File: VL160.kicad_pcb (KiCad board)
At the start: 4 copper layers, 24 x 14 mm, 12 parts, among them J1 USB_C_Receptacle, J2 USB3_A, U1 VL160, U2 LM3480-5.0

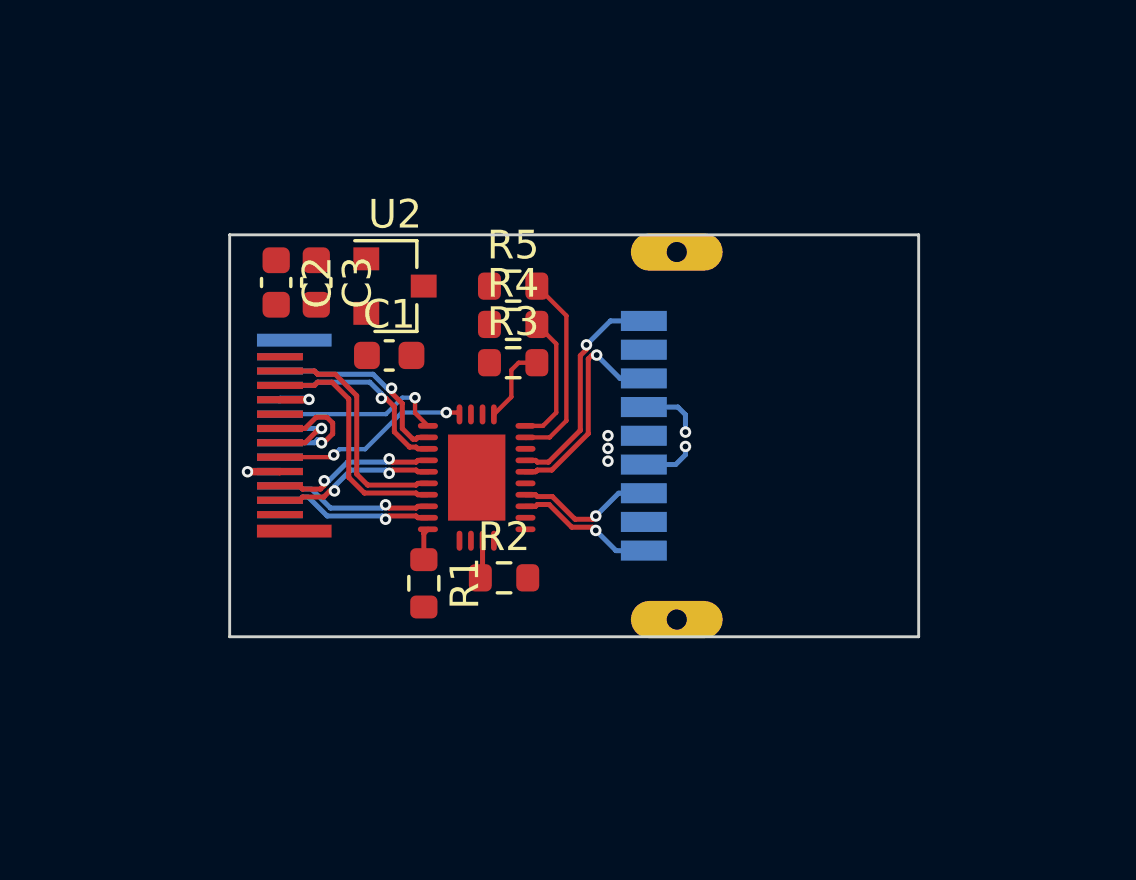
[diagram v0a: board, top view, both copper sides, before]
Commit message: Sync 2022/01/11 周二 21:14:02.89
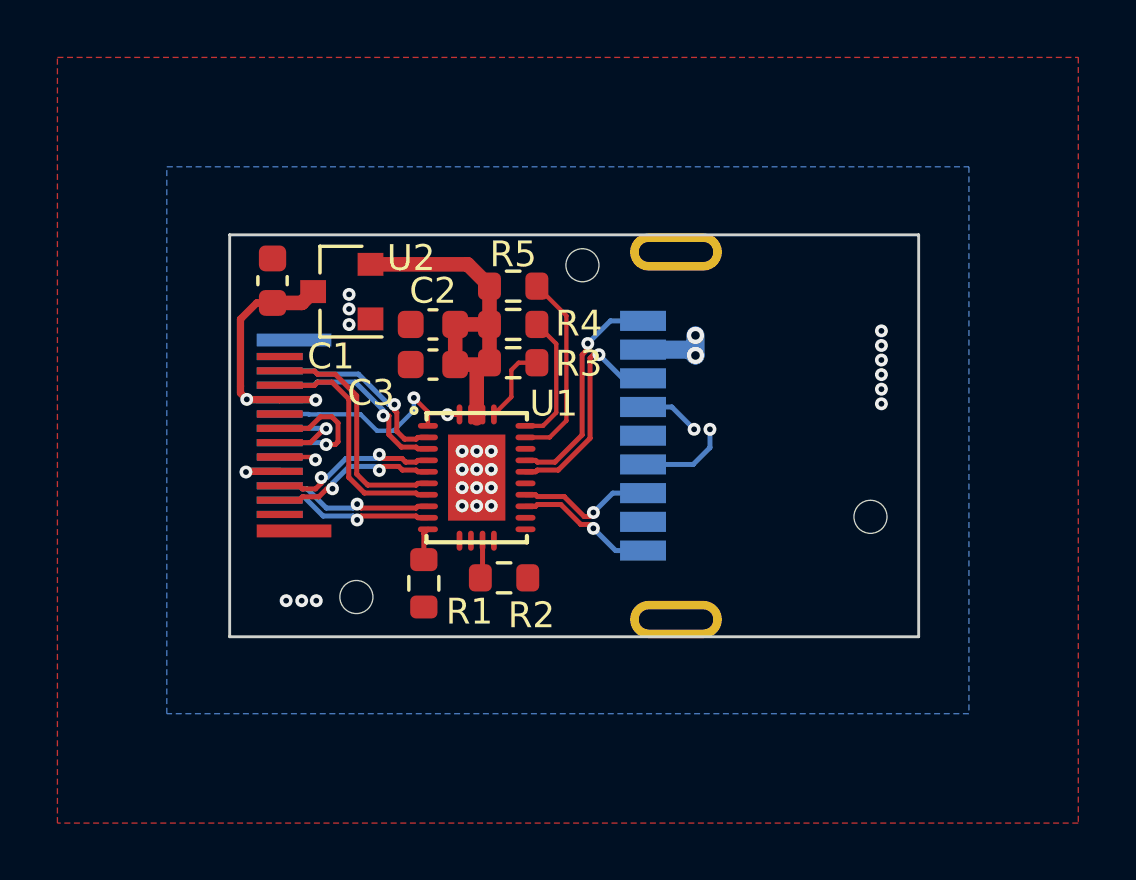
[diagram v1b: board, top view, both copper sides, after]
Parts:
- added H1: MountingHole, VL160:Hole_1.152mm_JLCSMT, F.Cu at (137.4, 102.6)
- added H2: MountingHole, VL160:Hole_1.152mm_JLCSMT, F.Cu at (155.3, 99.8)
- added H3: MountingHole, VL160:Hole_1.152mm_JLCSMT, F.Cu at (145.3, 91.1)
- J1, J2: moved to B.Cu
- U2: value LM3480-5.0 -> SE8550
- moved C2 5.65 mm to (140.1, 93.1), turned to 180 degrees
- moved C3 4.97 mm to (140.1, 94.5), turned to 180 degrees
- moved C1 4.83 mm to (134.5, 91.6), turned to 90 degrees
- moved J1 3.39 mm to (135.2, 93.6)
- moved U2 1.86 mm to (136.9, 92.0), turned to 180 degrees
- moved J2 1.47 mm to (148.7, 98.3), turned to 0 degrees
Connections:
- U1 pad 29: (no net) -> GND
- U2 pad 1: VCC -> GND
- U2 pad 2: VBUS -> VCC
- U2 pad 3: GND -> VBUS
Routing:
- net VBUS: track 8.71 -> 39.0 mm, vias 2 -> 5
- net VCC: track 0.00 -> 12.7 mm
- net /CC2: track 6.99 -> 8.77 mm
- net /CC1: track 6.11 -> 6.83 mm
- net GND: vias 1 -> 24
- net (no net): vias 2 -> 0
- added copper zone on B.Cu, net GND
- added copper zone on F.Cu, net GND
- added copper zone on In1.Cu, net GND
- added copper zone on In2.Cu, net GND
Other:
- net class 90R_IN: via_dia 0.4 -> 0.45
- net class 90R_OUT: via_dia 0.4 -> 0.45
- net class Default: via_dia 0.4 -> 0.45
- net class POWER: via_dia 0.5 -> 0.45; via_drill 0.3 -> 0.2
- rule via_min_drill: 0 -> 0.2
- rule via_min_size: 0 -> 0.45
